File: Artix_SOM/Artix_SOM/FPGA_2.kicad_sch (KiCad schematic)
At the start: 14 parts, among them SW1 SW_Push, U1 XC7A100T-FGG676

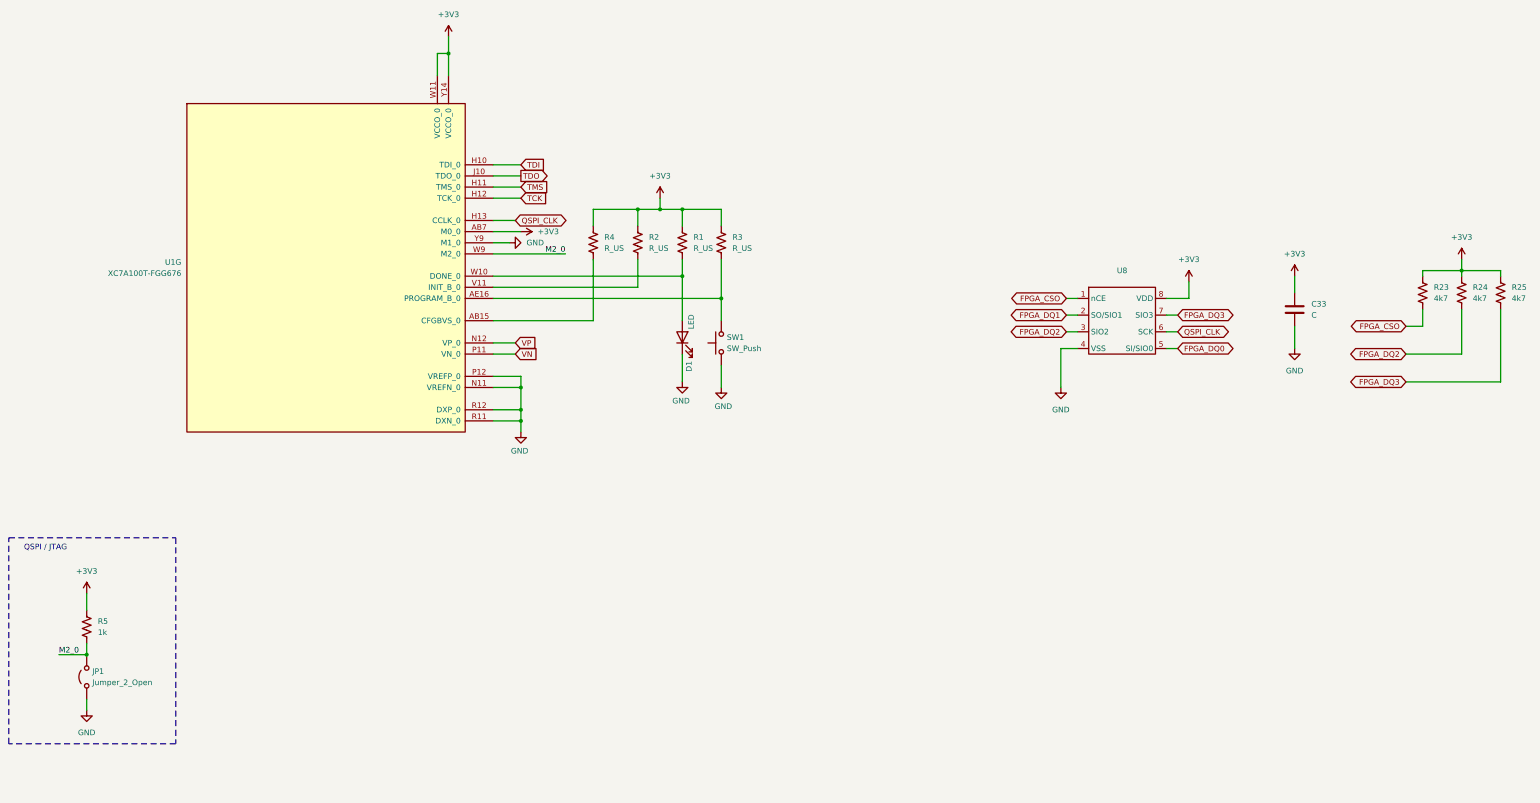
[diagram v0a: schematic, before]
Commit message: update
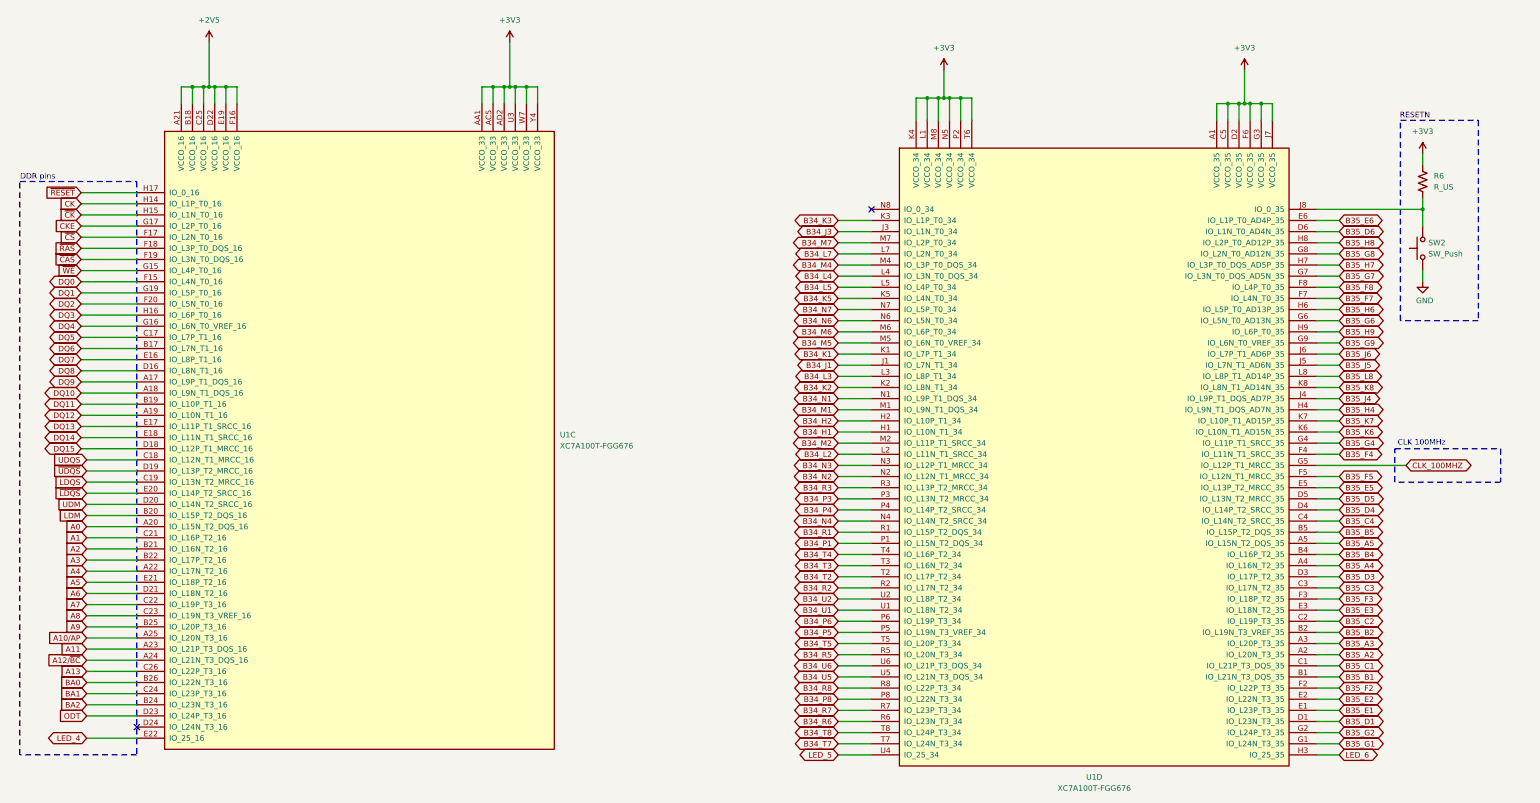
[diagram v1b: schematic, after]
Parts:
- removed C33: C, symbol Device:C
- removed D1: LED, symbol Device:LED
- removed JP1: Jumper_2_Open, symbol Jumper:Jumper_2_Open
- removed R1, R2, R3, R4: R_US, symbol Device:R_US
- removed R23, R24, R25: 4k7, symbol Device:R_US
- removed R5: 1k, symbol Device:R_US
- removed SW1: SW_Push, symbol Switch:SW_Push
- removed U1: XC7A100T-FGG676, symbol FPGA_Xilinx_Artix7:XC7A100T-FGG676
- removed U8: ~, symbol Sources:MT25QL128
- added R6: R_US, symbol Device:R_US
- added SW2: SW_Push, symbol Switch:SW_Push
- added U1: XC7A100T-FGG676, symbol FPGA_Xilinx_Artix7:XC7A100T-FGG676
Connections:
- net +3V3: now also R6.1, U1.A1 (VCCO_35), U1.AA1 (VCCO_33), U1.AC5 (VCCO_33), U1.AD2 (VCCO_33), U1.C5 (VCCO_35), U1.D2 (VCCO_35), U1.F6 (VCCO_35), U1.G3 (VCCO_35), U1.J7 (VCCO_35), U1.K4 (VCCO_34), U1.L1 (VCCO_34), U1.M8 (VCCO_34), U1.N5 (VCCO_34), U1.P2 (VCCO_34), U1.T6 (VCCO_34), U1.U3 (VCCO_33), U1.W7 (VCCO_33), U1.Y4 (VCCO_33)
- net GND: now also SW2.1
- new net: R6.2, SW2.2, U1.J8 (IO_0_35)
- new net +2V5: U1.A21 (VCCO_16), U1.B18 (VCCO_16), U1.C25 (VCCO_16), U1.D22 (VCCO_16), U1.E19 (VCCO_16), U1.F16 (VCCO_16)
- new net A0: U1.A20 (IO_L15N_T2_DQS_16)
- new net A1: U1.C21 (IO_L16P_T2_16)
- new net A10/AP: U1.A25 (IO_L20N_T3_16)
- new net A11: U1.A23 (IO_L21P_T3_DQS_16)
- new net A12/~{BC}: U1.A24 (IO_L21N_T3_DQS_16)
- new net A13: U1.C26 (IO_L22P_T3_16)
- new net A2: U1.B21 (IO_L16N_T2_16)
- new net A3: U1.B22 (IO_L17P_T2_16)
- new net A4: U1.A22 (IO_L17N_T2_16)
- new net A5: U1.E21 (IO_L18P_T2_16)
- new net A6: U1.D21 (IO_L18N_T2_16)
- new net A7: U1.C22 (IO_L19P_T3_16)
- new net A8: U1.C23 (IO_L19N_T3_VREF_16)
- new net A9: U1.B25 (IO_L20P_T3_16)
- new net B34_H1: U1.H1 (IO_L10N_T1_34)
- new net B34_H2: U1.H2 (IO_L10P_T1_34)
- new net B34_J1: U1.J1 (IO_L7N_T1_34)
- new net B34_J3: U1.J3 (IO_L1N_T0_34)
- new net B34_K1: U1.K1 (IO_L7P_T1_34)
- new net B34_K2: U1.K2 (IO_L8N_T1_34)
- new net B34_K3: U1.K3 (IO_L1P_T0_34)
- new net B34_K5: U1.K5 (IO_L4N_T0_34)
- new net B34_L2: U1.L2 (IO_L11N_T1_SRCC_34)
- new net B34_L3: U1.L3 (IO_L8P_T1_34)
- new net B34_L4: U1.L4 (IO_L3N_T0_DQS_34)
- new net B34_L5: U1.L5 (IO_L4P_T0_34)
- new net B34_L7: U1.L7 (IO_L2N_T0_34)
- new net B34_M1: U1.M1 (IO_L9N_T1_DQS_34)
- new net B34_M2: U1.M2 (IO_L11P_T1_SRCC_34)
- new net B34_M4: U1.M4 (IO_L3P_T0_DQS_34)
- new net B34_M5: U1.M5 (IO_L6N_T0_VREF_34)
- new net B34_M6: U1.M6 (IO_L6P_T0_34)
- new net B34_M7: U1.M7 (IO_L2P_T0_34)
- new net B34_N1: U1.N1 (IO_L9P_T1_DQS_34)
- new net B34_N2: U1.N2 (IO_L12N_T1_MRCC_34)
- new net B34_N3: U1.N3 (IO_L12P_T1_MRCC_34)
- new net B34_N4: U1.N4 (IO_L14N_T2_SRCC_34)
- new net B34_N6: U1.N6 (IO_L5N_T0_34)
- new net B34_N7: U1.N7 (IO_L5P_T0_34)
- new net B34_P1: U1.P1 (IO_L15N_T2_DQS_34)
- new net B34_P3: U1.P3 (IO_L13N_T2_MRCC_34)
- new net B34_P4: U1.P4 (IO_L14P_T2_SRCC_34)
- new net B34_P5: U1.P5 (IO_L19N_T3_VREF_34)
- new net B34_P6: U1.P6 (IO_L19P_T3_34)
- new net B34_P8: U1.P8 (IO_L22N_T3_34)
- new net B34_R1: U1.R1 (IO_L15P_T2_DQS_34)
- new net B34_R2: U1.R2 (IO_L17N_T2_34)
- new net B34_R3: U1.R3 (IO_L13P_T2_MRCC_34)
- new net B34_R5: U1.R5 (IO_L20N_T3_34)
- new net B34_R6: U1.R6 (IO_L23N_T3_34)
- new net B34_R7: U1.R7 (IO_L23P_T3_34)
- new net B34_R8: U1.R8 (IO_L22P_T3_34)
- new net B34_T2: U1.T2 (IO_L17P_T2_34)
- new net B34_T3: U1.T3 (IO_L16N_T2_34)
- new net B34_T4: U1.T4 (IO_L16P_T2_34)
- new net B34_T5: U1.T5 (IO_L20P_T3_34)
- new net B34_T7: U1.T7 (IO_L24N_T3_34)
- new net B34_T8: U1.T8 (IO_L24P_T3_34)
- new net B34_U1: U1.U1 (IO_L18N_T2_34)
- new net B34_U2: U1.U2 (IO_L18P_T2_34)
- new net B34_U5: U1.U5 (IO_L21N_T3_DQS_34)
- new net B34_U6: U1.U6 (IO_L21P_T3_DQS_34)
- new net B35_A2: U1.A2 (IO_L20N_T3_35)
- new net B35_A3: U1.A3 (IO_L20P_T3_35)
- new net B35_A4: U1.A4 (IO_L16N_T2_35)
- new net B35_A5: U1.A5 (IO_L15N_T2_DQS_35)
- new net B35_B1: U1.B1 (IO_L21N_T3_DQS_35)
- new net B35_B2: U1.B2 (IO_L19N_T3_VREF_35)
- new net B35_B4: U1.B4 (IO_L16P_T2_35)
- new net B35_B5: U1.B5 (IO_L15P_T2_DQS_35)
- new net B35_C1: U1.C1 (IO_L21P_T3_DQS_35)
- new net B35_C2: U1.C2 (IO_L19P_T3_35)
- new net B35_C3: U1.C3 (IO_L17N_T2_35)
- new net B35_C4: U1.C4 (IO_L14N_T2_SRCC_35)
- new net B35_D1: U1.D1 (IO_L23N_T3_35)
- new net B35_D3: U1.D3 (IO_L17P_T2_35)
- new net B35_D4: U1.D4 (IO_L14P_T2_SRCC_35)
- new net B35_D5: U1.D5 (IO_L13N_T2_MRCC_35)
- new net B35_D6: U1.D6 (IO_L1N_T0_AD4N_35)
- new net B35_E1: U1.E1 (IO_L23P_T3_35)
- new net B35_E2: U1.E2 (IO_L22N_T3_35)
- new net B35_E3: U1.E3 (IO_L18N_T2_35)
- new net B35_E5: U1.E5 (IO_L13P_T2_MRCC_35)
- new net B35_E6: U1.E6 (IO_L1P_T0_AD4P_35)
- new net B35_F2: U1.F2 (IO_L22P_T3_35)
- new net B35_F3: U1.F3 (IO_L18P_T2_35)
- new net B35_F4: U1.F4 (IO_L11N_T1_SRCC_35)
- new net B35_F5: U1.F5 (IO_L12N_T1_MRCC_35)
- new net B35_F7: U1.F7 (IO_L4N_T0_35)
- new net B35_F8: U1.F8 (IO_L4P_T0_35)
- new net B35_G1: U1.G1 (IO_L24N_T3_35)
- new net B35_G2: U1.G2 (IO_L24P_T3_35)
- new net B35_G4: U1.G4 (IO_L11P_T1_SRCC_35)
- new net B35_G6: U1.G6 (IO_L5N_T0_AD13N_35)
- new net B35_G7: U1.G7 (IO_L3N_T0_DQS_AD5N_35)
- new net B35_G8: U1.G8 (IO_L2N_T0_AD12N_35)
- new net B35_G9: U1.G9 (IO_L6N_T0_VREF_35)
- new net B35_H4: U1.H4 (IO_L9N_T1_DQS_AD7N_35)
- new net B35_H6: U1.H6 (IO_L5P_T0_AD13P_35)
- new net B35_H7: U1.H7 (IO_L3P_T0_DQS_AD5P_35)
- new net B35_H8: U1.H8 (IO_L2P_T0_AD12P_35)
- new net B35_H9: U1.H9 (IO_L6P_T0_35)
- new net B35_J4: U1.J4 (IO_L9P_T1_DQS_AD7P_35)
- new net B35_J5: U1.J5 (IO_L7N_T1_AD6N_35)
- new net B35_J6: U1.J6 (IO_L7P_T1_AD6P_35)
- new net B35_K6: U1.K6 (IO_L10N_T1_AD15N_35)
- new net B35_K7: U1.K7 (IO_L10P_T1_AD15P_35)
- new net B35_K8: U1.K8 (IO_L8N_T1_AD14N_35)
- new net B35_L8: U1.L8 (IO_L8P_T1_AD14P_35)
- new net BA0: U1.B26 (IO_L22N_T3_16)
- new net BA1: U1.C24 (IO_L23P_T3_16)
- new net BA2: U1.B24 (IO_L23N_T3_16)
- new net CK: U1.H14 (IO_L1P_T0_16)
- new net CKE: U1.G17 (IO_L2P_T0_16)
- new net CLK_100MHZ: U1.G5 (IO_L12P_T1_MRCC_35)
- new net DQ0: U1.F15 (IO_L4N_T0_16)
- new net DQ1: U1.G19 (IO_L5P_T0_16)
- new net DQ10: U1.A18 (IO_L9N_T1_DQS_16)
- new net DQ11: U1.B19 (IO_L10P_T1_16)
- new net DQ12: U1.A19 (IO_L10N_T1_16)
- new net DQ13: U1.E17 (IO_L11P_T1_SRCC_16)
- new net DQ14: U1.E18 (IO_L11N_T1_SRCC_16)
- new net DQ15: U1.D18 (IO_L12P_T1_MRCC_16)
- new net DQ2: U1.F20 (IO_L5N_T0_16)
- new net DQ3: U1.H16 (IO_L6P_T0_16)
- new net DQ4: U1.G16 (IO_L6N_T0_VREF_16)
- new net DQ5: U1.C17 (IO_L7P_T1_16)
- new net DQ6: U1.B17 (IO_L7N_T1_16)
- new net DQ7: U1.E16 (IO_L8P_T1_16)
- new net DQ8: U1.D16 (IO_L8N_T1_16)
- new net DQ9: U1.A17 (IO_L9P_T1_DQS_16)
- new net LDM: U1.B20 (IO_L15P_T2_DQS_16)
- new net LDQS: U1.C19 (IO_L13N_T2_MRCC_16)
- new net LED_4: U1.E22 (IO_25_16)
- new net LED_5: U1.U4 (IO_25_34)
- new net LED_6: U1.H3 (IO_25_35)
- new net ODT: U1.D23 (IO_L24P_T3_16)
- new net UDM: U1.D20 (IO_L14N_T2_SRCC_16)
- new net UDQS: U1.C18 (IO_L12N_T1_MRCC_16)
- new net ~{CAS}: U1.F19 (IO_L3N_T0_DQS_16)
- new net ~{CK}: U1.H15 (IO_L1N_T0_16)
- new net ~{CS}: U1.F17 (IO_L2N_T0_16)
- new net ~{LDQS}: U1.E20 (IO_L14P_T2_SRCC_16)
- new net ~{RAS}: U1.F18 (IO_L3P_T0_DQS_16)
- new net ~{RESET}: U1.H17 (IO_0_16)
- new net ~{UDQS}: U1.D19 (IO_L13P_T2_MRCC_16)
- new net ~{WE}: U1.G15 (IO_L4P_T0_16)
- no-connect marks 0 -> 2
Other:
- note added: "CLK 100MHz"
- note added: "DDR pins"
- note added: "RESETN"
- note removed: "QSPI / JTAG"
